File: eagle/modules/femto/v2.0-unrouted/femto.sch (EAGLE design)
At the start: 29 parts, among them IC1 MEGA8-AI, J1 RJ12RIGHTANGLE-I2C, J2 RJ12RIGHTANGLE-I2C

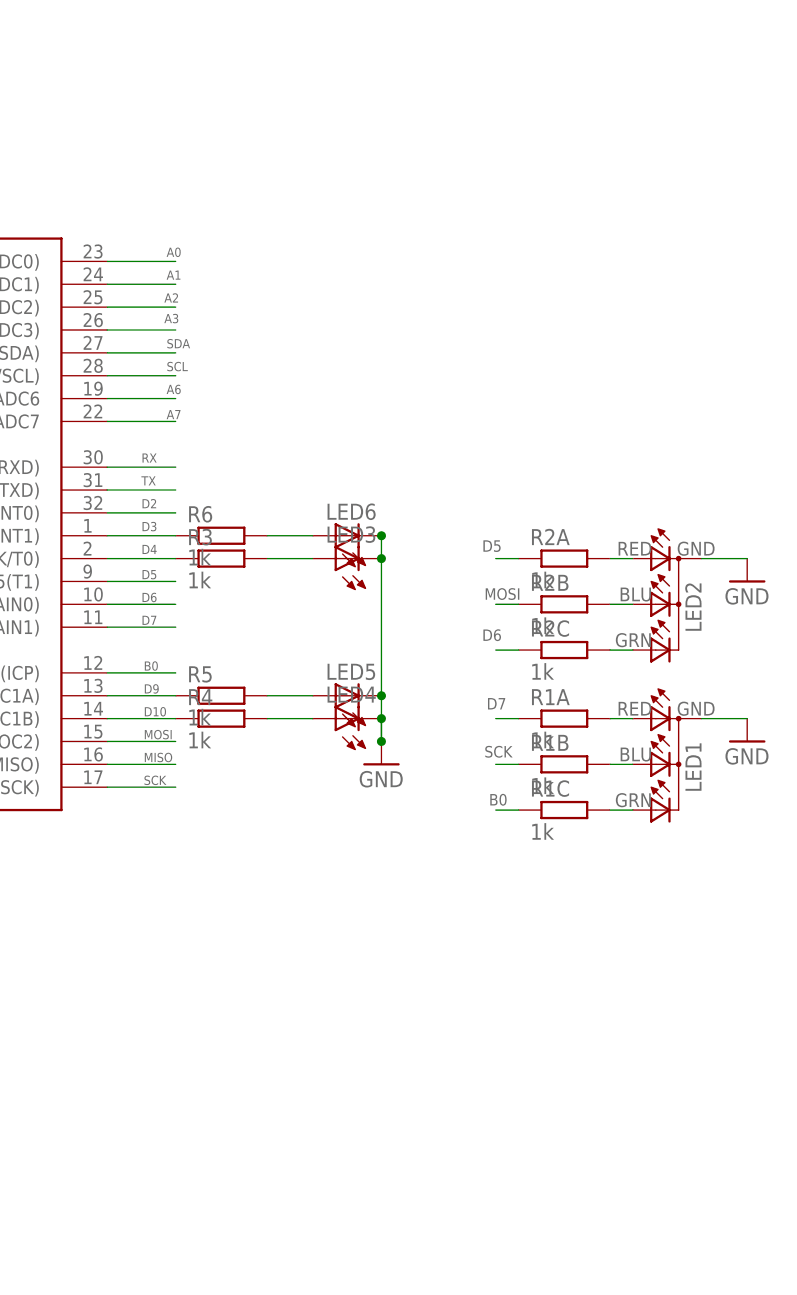
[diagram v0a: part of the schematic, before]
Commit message: Update femto
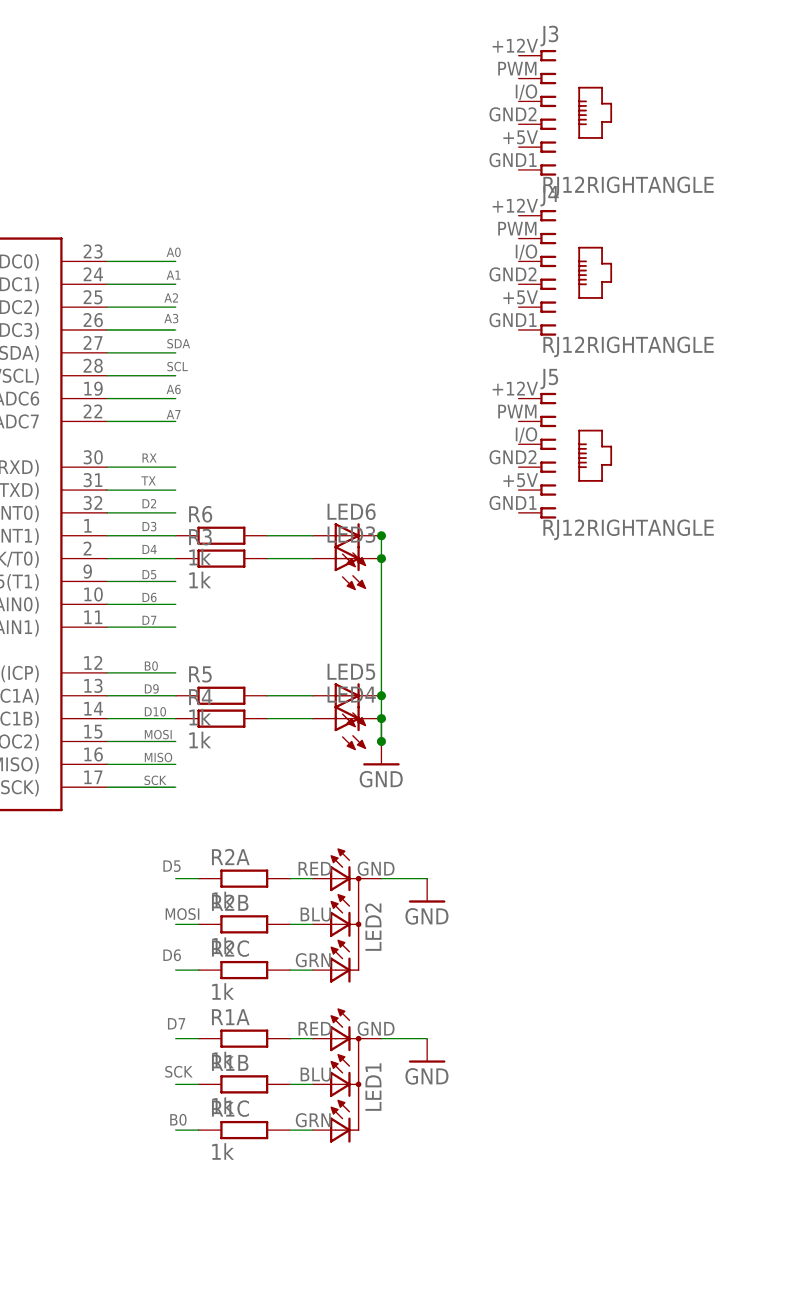
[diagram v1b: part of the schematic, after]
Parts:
- added J3, J4, J5: RJ12RIGHTANGLE, lpatiny:RJ12RIGHTANGLE
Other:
- moved on the sheet: LED1, LED2, R1A, R1B, R1C, R2A, R2B, R2C
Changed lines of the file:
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@@
 <?xml version="1.0" encoding="utf-8"?>
 <!DOCTYPE eagle SYSTEM "eagle.dtd">
-<eagle version="6.4">
+<eagle version="6.1">
 <drawing>
 <settings>
@@
 <part name="R3" library="resistor" deviceset="R-EU_" device="M1206" value="1k"/>
 <part name="LED3" library="lpatiny" deviceset="LED3MM" device=""/>
+<part name="J3" library="lpatiny" deviceset="RJ12" device="RIGHTANGLE"/>
+<part name="J4" library="lpatiny" deviceset="RJ12" device="RIGHTANGLE"/>
+<part name="J5" library="lpatiny" deviceset="RJ12" device="RIGHTANGLE"/>
 </parts>
 <sheets>
@@
 <instance part="J2" gate="G$1" x="7.62" y="-33.02"/>
 <instance part="C3" gate="G$1" x="0" y="33.02" rot="R180"/>
-<instance part="LED2" gate="G$1" x="147.32" y="30.48" rot="R270"/>
-<instance part="LED1" gate="G$1" x="147.32" y="12.7" rot="R270"/>
-<instance part="R2A" gate="G$1" x="134.62" y="35.56"/>
-<instance part="R2B" gate="G$1" x="134.62" y="30.48"/>
-<instance part="R2C" gate="G$1" x="134.62" y="25.4"/>
-<instance part="R1A" gate="G$1" x="134.62" y="17.78"/>
-<instance part="R1B" gate="G$1" x="134.62" y="12.7"/>
-<instance part="R1C" gate="G$1" x="134.62" y="7.62"/>
-<instance part="GND7" gate="1" x="154.94" y="33.02"/>
-<instance part="GND8" gate="1" x="154.94" y="15.24"/>
+<instance part="LED2" gate="G$1" x="111.76" y="-5.08" rot="R270"/>
+<instance part="LED1" gate="G$1" x="111.76" y="-22.86" rot="R270"/>
+<instance part="R2A" gate="G$1" x="99.06" y="0"/>
+<instance part="R2B" gate="G$1" x="99.06" y="-5.08"/>
+<instance part="R2C" gate="G$1" x="99.06" y="-10.16"/>
+<instance part="R1A" gate="G$1" x="99.06" y="-17.78"/>
+<instance part="R1B" gate="G$1" x="99.06" y="-22.86"/>
+<instance part="R1C" gate="G$1" x="99.06" y="-27.94"/>
+<instance part="GND7" gate="1" x="119.38" y="-2.54"/>
+<instance part="GND8" gate="1" x="119.38" y="-20.32"/>
 <instance part="GND3" gate="1" x="114.3" y="12.7"/>
 <instance part="R6" gate="G$1" x="96.52" y="38.1"/>
@@
 <instance part="R3" gate="G$1" x="96.52" y="35.56"/>
 <instance part="LED3" gate="G$1" x="109.22" y="35.56" rot="R90"/>
+<instance part="J3" gate="G$1" x="132.08" y="86.36"/>
+<instance part="J4" gate="G$1" x="132.08" y="68.58"/>
+<instance part="J5" gate="G$1" x="132.08" y="48.26"/>
 </instances>
 <busses>
@@
 <segment>
 <pinref part="LED2" gate="G$1" pin="A2"/>
-<wire x1="149.86" y1="35.56" x2="154.94" y2="35.56" width="0.1524" layer="91"/>
+<wire x1="114.3" y1="0" x2="119.38" y2="0" width="0.1524" layer="91"/>
 <pinref part="GND7" gate="1" pin="GND"/>
 </segment>
 <segment>
 <pinref part="LED1" gate="G$1" pin="A2"/>
-<wire x1="149.86" y1="17.78" x2="154.94" y2="17.78" width="0.1524" layer="91"/>
+<wire x1="114.3" y1="-17.78" x2="119.38" y2="-17.78" width="0.1524" layer="91"/>
 <pinref part="GND8" gate="1" pin="GND"/>
 </segment>
@@
 <segment>
 <pinref part="R1B" gate="G$1" pin="1"/>
-<wire x1="129.54" y1="12.7" x2="127" y2="12.7" width="0.1524" layer="91"/>
-<label x="125.73" y="13.462" size="1.27" layer="95"/>
+<wire x1="93.98" y1="-22.86" x2="91.44" y2="-22.86" width="0.1524" layer="91"/>
+<label x="90.17" y="-22.098" size="1.27" layer="95"/>
 </segment>
 <segment>
@@
 <segment>
 <pinref part="R2B" gate="G$1" pin="1"/>
-<wire x1="129.54" y1="30.48" x2="127" y2="30.48" width="0.1524" layer="91"/>
-<label x="125.73" y="30.988" size="1.27" layer="95"/>
+<wire x1="93.98" y1="-5.08" x2="91.44" y2="-5.08" width="0.1524" layer="91"/>
+<label x="90.17" y="-4.572" size="1.27" layer="95"/>
 </segment>
 <segment>
@@
 <pinref part="R2A" gate="G$1" pin="2"/>
 <pinref part="LED2" gate="G$1" pin="CRED"/>
-<wire x1="142.24" y1="35.56" x2="139.7" y2="35.56" width="0.1524" layer="91"/>
+<wire x1="106.68" y1="0" x2="104.14" y2="0" width="0.1524" layer="91"/>
 </segment>
 </net>
@@
 <pinref part="LED2" gate="G$1" pin="CBLUE"/>
 <pinref part="R2B" gate="G$1" pin="2"/>
-<wire x1="142.24" y1="30.48" x2="139.7" y2="30.48" width="0.1524" layer="91"/>
+<wire x1="106.68" y1="-5.08" x2="104.14" y2="-5.08" width="0.1524" layer="91"/>
 </segment>
 </net>
@@
 <pinref part="R2C" gate="G$1" pin="2"/>
 <pinref part="LED2" gate="G$1" pin="CGREEN"/>
-<wire x1="142.24" y1="25.4" x2="139.7" y2="25.4" width="0.1524" layer="91"/>
+<wire x1="106.68" y1="-10.16" x2="104.14" y2="-10.16" width="0.1524" layer="91"/>
 </segment>
 </net>
@@
 <pinref part="LED1" gate="G$1" pin="CRED"/>
 <pinref part="R1A" gate="G$1" pin="2"/>
-<wire x1="142.24" y1="17.78" x2="139.7" y2="17.78" width="0.1524" layer="91"/>
+<wire x1="106.68" y1="-17.78" x2="104.14" y2="-17.78" width="0.1524" layer="91"/>
 </segment>
 </net>
@@
 <pinref part="R1B" gate="G$1" pin="2"/>
 <pinref part="LED1" gate="G$1" pin="CBLUE"/>
-<wire x1="142.24" y1="12.7" x2="139.7" y2="12.7" width="0.1524" layer="91"/>
+<wire x1="106.68" y1="-22.86" x2="104.14" y2="-22.86" width="0.1524" layer="91"/>
 </segment>
 </net>
@@
 <pinref part="LED1" gate="G$1" pin="CGREEN"/>
 <pinref part="R1C" gate="G$1" pin="2"/>
-<wire x1="142.24" y1="7.62" x2="139.7" y2="7.62" width="0.1524" layer="91"/>
+<wire x1="106.68" y1="-27.94" x2="104.14" y2="-27.94" width="0.1524" layer="91"/>
 </segment>
 </net>
@@
 <segment>
 <pinref part="R2A" gate="G$1" pin="1"/>
-<wire x1="129.54" y1="35.56" x2="127" y2="35.56" width="0.1524" layer="91"/>
-<label x="125.476" y="36.322" size="1.27" layer="95"/>
+<wire x1="93.98" y1="0" x2="91.44" y2="0" width="0.1524" layer="91"/>
+<label x="89.916" y="0.762" size="1.27" layer="95"/>
 </segment>
 <segment>
@@
 <segment>
 <pinref part="R2C" gate="G$1" pin="1"/>
-<wire x1="129.54" y1="25.4" x2="127" y2="25.4" width="0.1524" layer="91"/>
-<label x="125.476" y="26.416" size="1.27" layer="95"/>
+<wire x1="93.98" y1="-10.16" x2="91.44" y2="-10.16" width="0.1524" layer="91"/>
+<label x="89.916" y="-9.144" size="1.27" layer="95"/>
 </segment>
 </net>
@@
 <segment>
 <pinref part="R1A" gate="G$1" pin="1"/>
-<wire x1="129.54" y1="17.78" x2="127" y2="17.78" width="0.1524" layer="91"/>
-<label x="125.984" y="18.796" size="1.27" layer="95"/>
+<wire x1="93.98" y1="-17.78" x2="91.44" y2="-17.78" width="0.1524" layer="91"/>
+<label x="90.424" y="-16.764" size="1.27" layer="95"/>
 </segment>
 <segment>
@@
 <segment>
 <pinref part="R1C" gate="G$1" pin="1"/>
-<wire x1="129.54" y1="7.62" x2="127" y2="7.62" width="0.1524" layer="91"/>
-<label x="126.238" y="8.128" size="1.27" layer="95"/>
-</segment>
-</net>
+<wire x1="93.98" y1="-27.94" x2="91.44" y2="-27.94" width="0.1524" layer="91"/>
+<label x="90.678" y="-27.432" size="1.27" layer="95"/>
+</segment>
+</net>
